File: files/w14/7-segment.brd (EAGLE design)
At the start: 100 x 80 mm, 16 parts

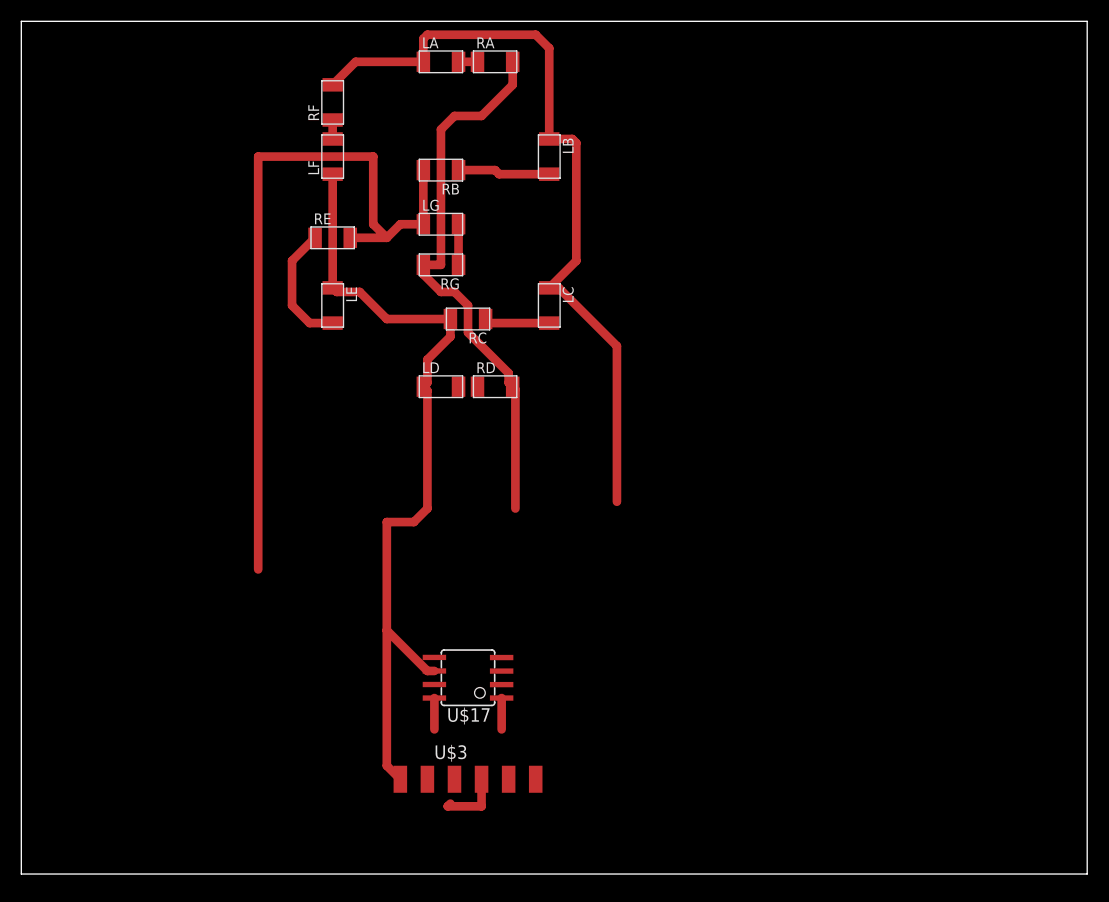
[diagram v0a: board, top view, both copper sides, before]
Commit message: board programmed
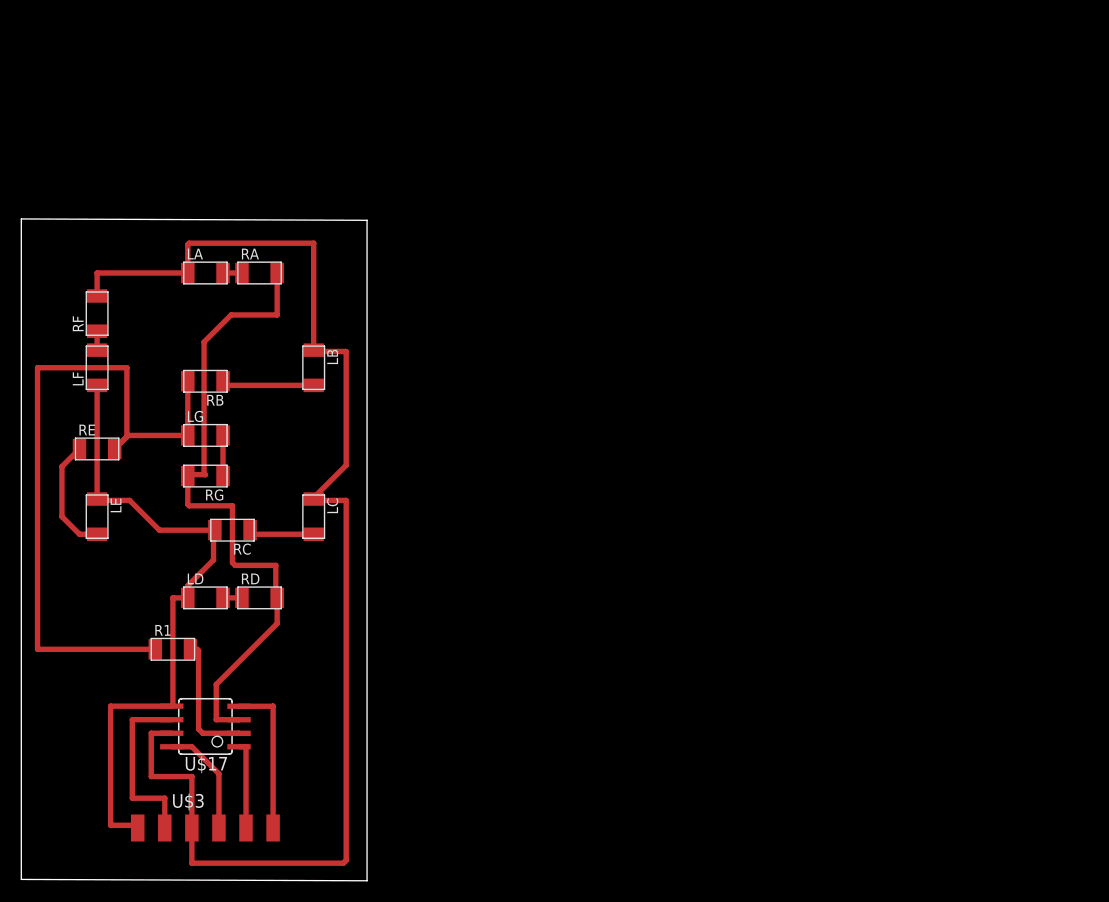
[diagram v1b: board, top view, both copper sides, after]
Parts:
- added R1: 0, fab:R1206FAB
- moved LB 29.7 mm to (27.4, 47.5)
- moved LC 29.7 mm to (27.4, 33.5)
- moved RA 29.7 mm to (22.4, 56.4)
- moved LA 29.7 mm to (17.3, 56.4)
- moved LE 29.7 mm to (7.11, 33.5)
- moved LF 29.7 mm to (7.11, 47.5)
- moved RB 29.7 mm to (17.3, 46.2)
- moved RD 29.7 mm to (22.4, 25.9)
- moved LD 29.7 mm to (17.3, 25.9)
- moved LG 29.7 mm to (17.3, 41.1)
- moved RC 29.7 mm to (19.8, 32.3)
- moved RE 29.7 mm to (7.11, 39.9)
- moved RF 29.7 mm to (7.11, 52.6)
- moved RG 29.7 mm to (17.3, 37.3)
- moved U$17 25.1 mm to (17.3, 13.8)
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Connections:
- net MISO: now also U$3.5; no longer LD.1, LE.1, LF.1, RC.2, U$3.6
- net MOSI: now also LD.1, LE.1, LF.1, RC.2, U$3.6; no longer U$3.5
- net PB3: now also R1.1, R1.2
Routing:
- net MOSI: track 0.00 -> 61.8 mm
- net MISO: track 77.0 -> 16.9 mm
- net SCK: track 73.1 -> 122.8 mm
- net GND: track 0.00 -> 14.6 mm
- net PB4: track 52.2 -> 61.3 mm
- net PB3: track 70.1 -> 78.5 mm
- net RST: track 2.94 -> 8.28 mm
- net N$6: track 0.00 -> 1.78 mm
- net VCC: track 9.02 -> 10.6 mm
- net N$7: track 11.7 -> 11.0 mm
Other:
- board size 100 x 80 mm -> 32.4 x 62.1 mm
